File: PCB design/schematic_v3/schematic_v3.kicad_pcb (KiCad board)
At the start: 4 copper layers, 67 x 43 mm, 117 parts, among them IC1 LAN9252, J1 Conn_01x04_Pin, J2 Conn_01x02_Pin, J3 connection_moteur, J4 Conn_01x05_Pin, J5 Conn_01x03_Pin, Q1 AO3400A, U1 SP3485CN, U2 HX1188NL, U3 24FC512-I/ST, U4 LMR14030SQDPRTQ1, U5 STM32F446RETx, U6 AP63203WU, Y1 25MHz, Y2 8MHz

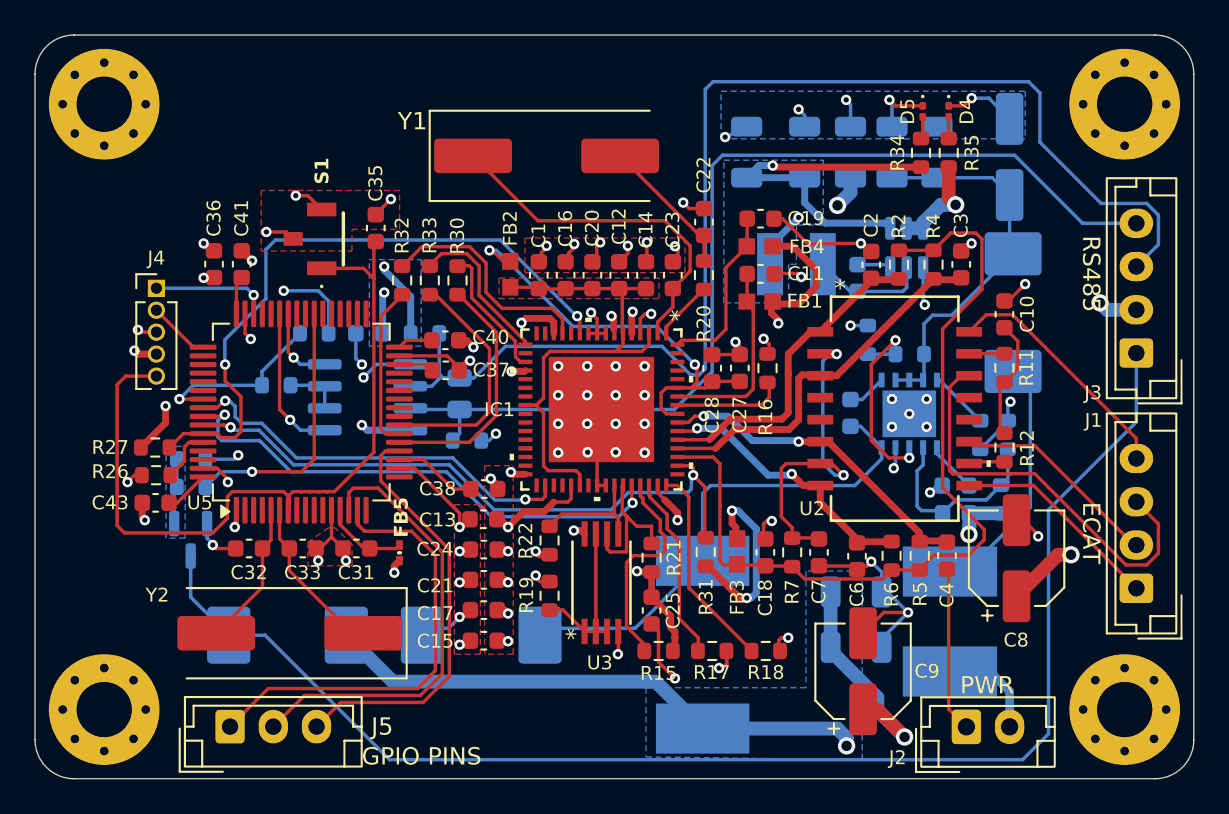
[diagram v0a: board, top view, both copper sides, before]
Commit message: PCB ordered
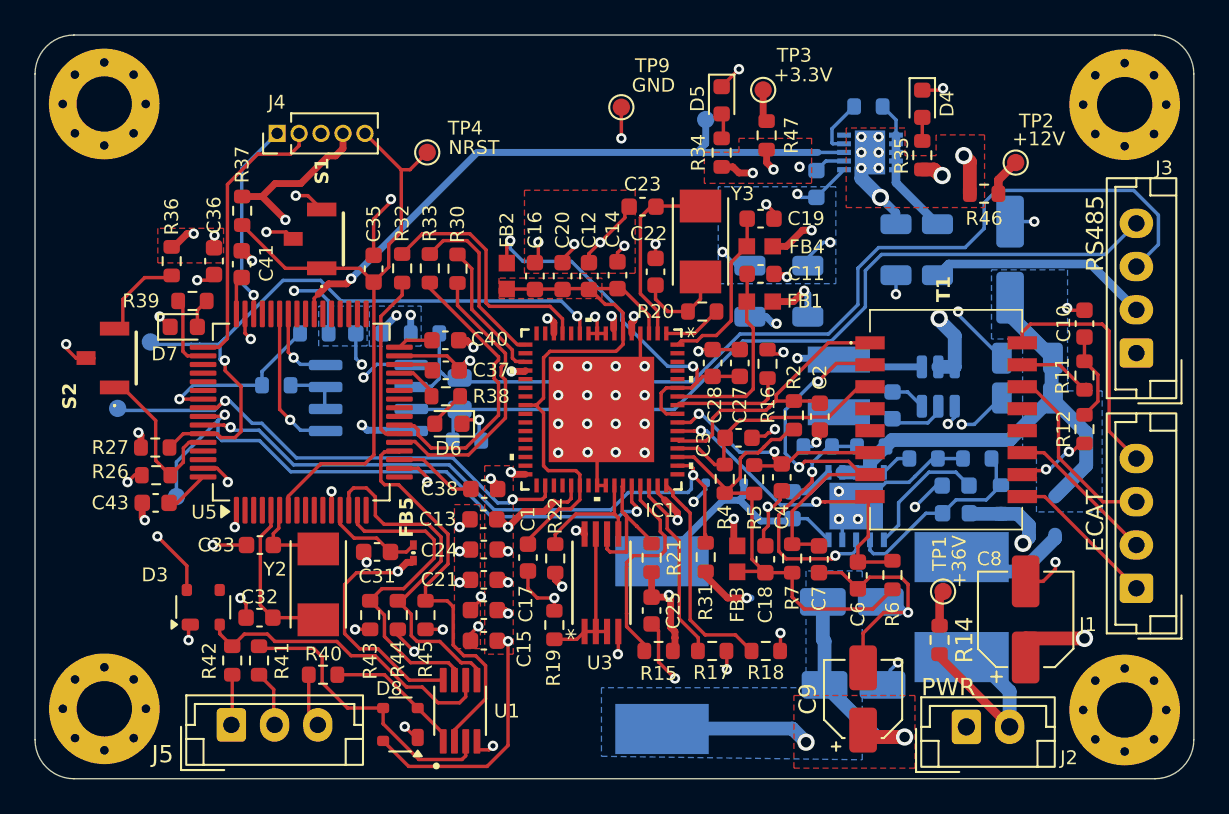
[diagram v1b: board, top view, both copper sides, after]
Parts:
- removed Q1: AO3400A, Package_TO_SOT_SMD:SOT-23
- removed U2: HX1188NL, footprints:HX1188NL
- removed Y1: 25MHz, Crystal:Crystal_SMD_HC49-SD
- added C50: 10u, Capacitor_SMD:C_1206_3216Metric, B.Cu at (175.7, 88.6)
- added C51: 56p, Capacitor_SMD:C_0603_1608Metric, B.Cu at (168.7, 84.8)
- added D6: LED_Small, LED_SMD:LED_0603_1608Metric, F.Cu at (147.4, 98.7)
- added D7: LED_Small, LED_SMD:LED_0603_1608Metric, F.Cu at (132.1, 93.1)
- added D8: PRTR5V0U2X, Package_TO_SOT_SMD:SOT-143, F.Cu at (144.6, 116.1)
- added IC2: SON50P300X300X100-11N-D, footprints:MP5000ADQ-LF-Z, B.Cu at (171.8, 83.0)
- added R36: 1k, Resistor_SMD:R_0603_1608Metric, F.Cu at (131.4, 89.3)
- added R37: 10k, Resistor_SMD:R_0603_1608Metric, F.Cu at (135.5, 86.4)
- added R38: 1k, Resistor_SMD:R_0603_1608Metric, F.Cu at (147.3, 97.1)
- added R39: 1k, Resistor_SMD:R_0603_1608Metric, F.Cu at (132.6, 91.6)
- added R40: 1k, Resistor_SMD:R_0603_1608Metric, F.Cu at (140.2, 113.2)
- added R41: 1k, Resistor_SMD:R_0603_1608Metric, F.Cu at (136.5, 112.4)
- added R42: 1k, Resistor_SMD:R_0603_1608Metric, F.Cu at (134.9, 112.4)
- added R43: 10k, Resistor_SMD:R_0603_1608Metric, F.Cu at (142.9, 109.8)
- added R44: 10k, Resistor_SMD:R_0603_1608Metric, F.Cu at (144.5, 109.8)
- added R45: 10k, Resistor_SMD:R_0603_1608Metric, F.Cu at (146.1, 109.8)
- added R46: 100, Resistor_SMD:R_0603_1608Metric, F.Cu at (178.4, 85.4)
- added R47: 100, Resistor_SMD:R_0603_1608Metric, F.Cu at (165.8, 82.0)
- added S2: B3U-1100PM, footprints:B3U1100PM, F.Cu at (128.1, 94.9)
- added T1: 7490100110A, footprints:7490100110A, F.Cu at (176.0, 98.5)
- added TP1: TestPoint, TestPoint:TestPoint_Pad_D1.0mm, F.Cu at (176.0, 108.4)
- added TP2: TestPoint, TestPoint:TestPoint_Pad_D1.0mm, F.Cu at (180.2, 83.6)
- added TP3: TestPoint, TestPoint:TestPoint_Pad_D1.0mm, F.Cu at (165.6, 79.4)
- added TP4: TestPoint, TestPoint:TestPoint_Pad_D1.0mm, F.Cu at (146.2, 83.0)
- added TP5: TestPoint, TestPoint:TestPoint_Pad_D1.0mm, B.Cu at (130.2, 94.0)
- added TP6: TestPoint, TestPoint:TestPoint_Pad_D1.0mm, B.Cu at (131.7, 102.9)
- added TP7: TestPoint, TestPoint:TestPoint_Pad_D1.0mm, B.Cu at (128.3, 97.8)
- added TP8: TestPoint, TestPoint:TestPoint_Pad_D1.0mm, B.Cu at (162.3, 81.1)
- added TP9: TestPoint, TestPoint:TestPoint_Pad_D1.0mm, F.Cu at (157.4, 80.4)
- added U7: MAX3485, Package_SO:SOIC-8_3.9x4.9mm_P1.27mm, B.Cu at (142.8, 97.2)
- added Y3: ABM3-25.000MHZ-D2Y-T, footprints:ABM3-25.000MHZ-D2Y-T, F.Cu at (162.0, 88.2)
- C32, C33: value 20p -> 27p
- C46, C48: footprint Capacitor_SMD:C_1206_3216Metric -> Capacitor_SMD:C_Elec_4x5.8
- C8: value 47u -> 10u
- C9: value 47u -> 1u; footprint Capacitor_SMD:CP_Elec_5x5.4 -> Capacitor_SMD:CP_Elec_4x5.4
- D1, D2: value B340 -> PMEG3020EJ; footprint Diode_SMD:D_SMC -> Diode_SMD:D_SOD-323F
- D3: value B340 -> PRTR5V0U2X; footprint Diode_SMD:D_SMC -> Package_TO_SOT_SMD:SOT-143; moved to F.Cu
- D4, D5: footprint LED_SMD:LED_0201_0603Metric -> LED_SMD:LED_0603_1608Metric
- R14: value 10k -> 100; moved to F.Cu
- R16: value 12k -> 12.1k
- R21, R22: value 2k -> 1k
- U1: value SP3485CN -> SN74LVC3G17DCTRE4; footprint Package_SO:SOIC-8_3.9x4.9mm_P1.27mm -> footprints:SN74LVC3G17DCTRE4; moved to F.Cu
- Y2: value 8MHz -> ABM3-20.000MHZ-D2Y-T; footprint Crystal:Crystal_SMD_HC49-SD -> footprints:ABM3-20.000MHZ-D2Y-T
- moved H3 68.6 mm to (186.5, 80.2), turned to 0 degrees
- moved H2 59.0 mm to (127.5, 115.2), turned to 0 degrees
- moved D1 44.9 mm to (182.5, 104.0), turned to -90 degrees
- moved R13 44.9 mm to (171.7, 80.4)
- moved R14 44.5 mm to (175.8, 111.2), turned to -90 degrees
- moved H4 35.0 mm to (186.5, 115.2), turned to 0 degrees
- moved D2 19.4 mm to (163.4, 102.1), turned to 180 degrees
- moved U1 18.9 mm to (148.1, 115.3), turned to 90 degrees
- moved R4 17.3 mm to (163.4, 101.9), turned to 90 degrees
- moved C1 16.3 mm to (152.0, 106.4), turned to 90 degrees
- moved C3 16.3 mm to (164.2, 99.5), turned to 0 degrees
- moved C30 16.2 mm to (180.9, 97.2), turned to 180 degrees
- moved D3 16.2 mm to (133.2, 109.3), turned to 90 degrees
- moved C29 13.0 mm to (180.9, 94.9), turned to 180 degrees
- moved D5 11.6 mm to (163.2, 80.0)
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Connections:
- net /TCT renamed /RCT
- C10 pad 2: GND -> GNDREF
- C42 pad 2: Net-(D3-K) -> Net-(D2-K)
- D1 pad 1: +12V -> /VIN
- D1 pad 2: /DRAIN -> Net-(D1-A)
- D2 pad 1: /VIN -> Net-(D2-K)
- D2 pad 2: Net-(D2-A) -> GND
- D3 pad 1: Net-(D3-K) -> GND
- D3 pad 2: GND -> Net-(D3-I/O1)
- F1 pad 2: Net-(D2-A) -> Net-(D1-A)
- J3 pad 1: /DRAIN -> GND
- J3 pad 2: +12V -> Net-(J3-Pin_2)
- J5 pad 1: /PA1 -> Net-(J5-Pin_1)
- J5 pad 2: /PA0 -> Net-(J5-Pin_2)
- J5 pad 3: /PA4 -> Net-(J5-Pin_3)
- L1 pad 1: Net-(D3-K) -> Net-(D2-K)
- R13 pad 1: /GATE -> Net-(IC2-I-LIMIT)
- R13 pad 2: /ALIM_MOTOR -> Net-(IC2-SOURCE_1)
- R14 pad 1: GND -> Net-(R14-Pad1)
- R14 pad 2: /GATE -> +36V
- U1 pad 1: /RO -> Net-(D8-I/O1)
- U1 pad 2: /DE/RE -> /PA4
- U1 pad 3: /DE/RE -> Net-(D8-I/O2)
- U1 pad 4: /DI -> GND
- U1 pad 5: GND -> /PA0
- U1 pad 6: /DATA+ -> Net-(D3-I/O1)
- U1 pad 7: /DATA- -> /PA1
- U4 pad 10: Net-(D3-K) -> Net-(D2-K)
- U5 pad 29: unconnected-(U5-PB10-Pad29) -> /PB10
- U5 pad 50: unconnected-(U5-PA15-Pad50) -> /PA15
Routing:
- net /DRAIN: track 80.6 -> 0.00 mm
- net Net-(D3-K): track 29.1 -> 0.00 mm
- net +12V: track 62.4 -> 39.7 mm, vias 7 -> 14
- net /VDD33TXRX1: track 49.5 -> 27.5 mm
- net /ALIM_MOTOR: track 15.4 -> 37.4 mm
- net Net-(D3-I/O1): track 0.00 -> 17.8 mm
- net Net-(D8-I/O2): track 0.00 -> 16.7 mm
- net /DATA+: track 72.4 -> 57.1 mm
- net Net-(D2-A): track 14.5 -> 0.00 mm
- net /TX_N: track 24.4 -> 10.8 mm
- net +3.3V: track 89.7 -> 103.2 mm, vias 31 -> 37
- net Net-(D2-K): track 0.00 -> 13.1 mm
- net Net-(J3-Pin_2): track 0.00 -> 12.9 mm
- net /SWCLK: track 3.59 -> 16.3 mm
- net /OSCO: track 20.6 -> 10.9 mm
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- added copper zone on F.Cu, net +12V
- added copper zone on B.Cu, net /VIN
- added copper zone on In1.Cu, net GNDREF
- removed copper zone on B.Cu, net /GATE
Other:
- board text added: "+12V"
- board text added: "+36V"
- board text added: "ALIM_MOTOR"
- board text added: "IRQ"
- board text added: "RST#"
- board text added: "SYNC0"
- board text removed: "GPIO PINS"
